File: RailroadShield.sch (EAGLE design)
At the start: 70 parts, among them J1 5520250-3, J2 5520250-3, J3 5520250-3, J4 5520426-4, J5 5520426-4, J6 KK-156-5, J7 KK-156-5, J8 MSTB-02, Q1 PMBT2222, U1 LM393M, U2 MCP2515-ST, U3 MCP2551-SN, U4 MAX3468CSA, U5 MAX3468CSA, U6 MAX3468CSA, U7 LM317LCDR, U8 6N137SD, Y1 16Mhz

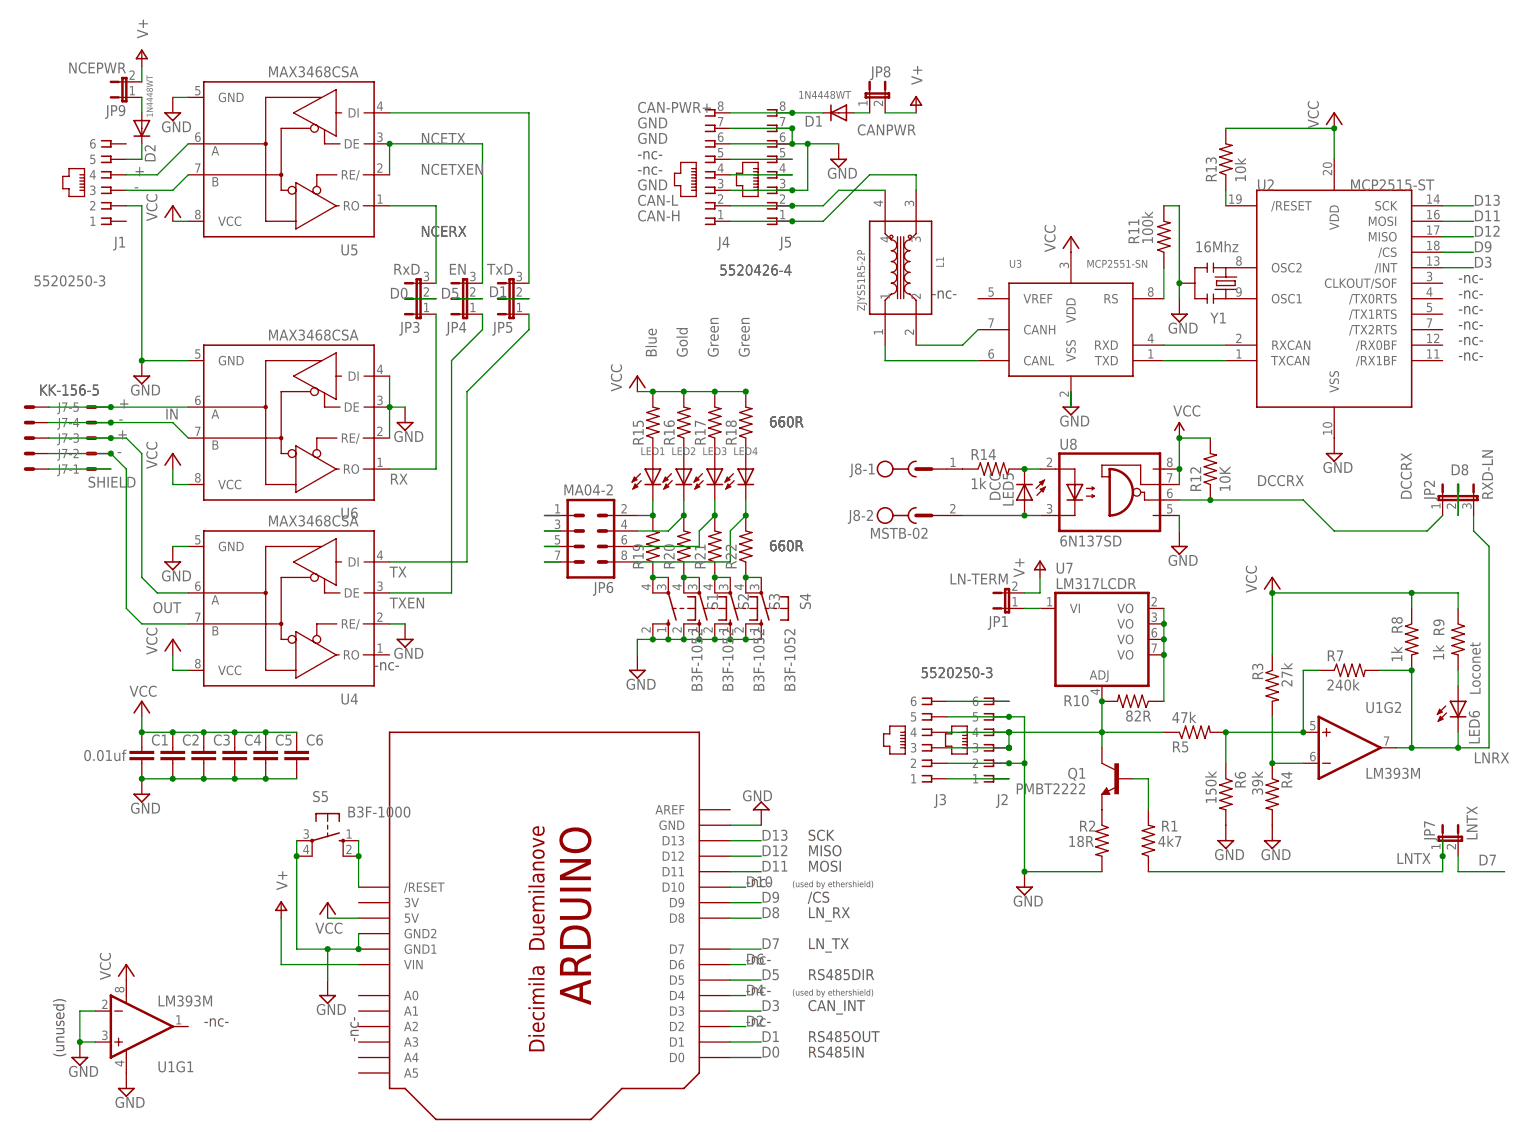
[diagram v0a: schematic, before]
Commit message: 2.3
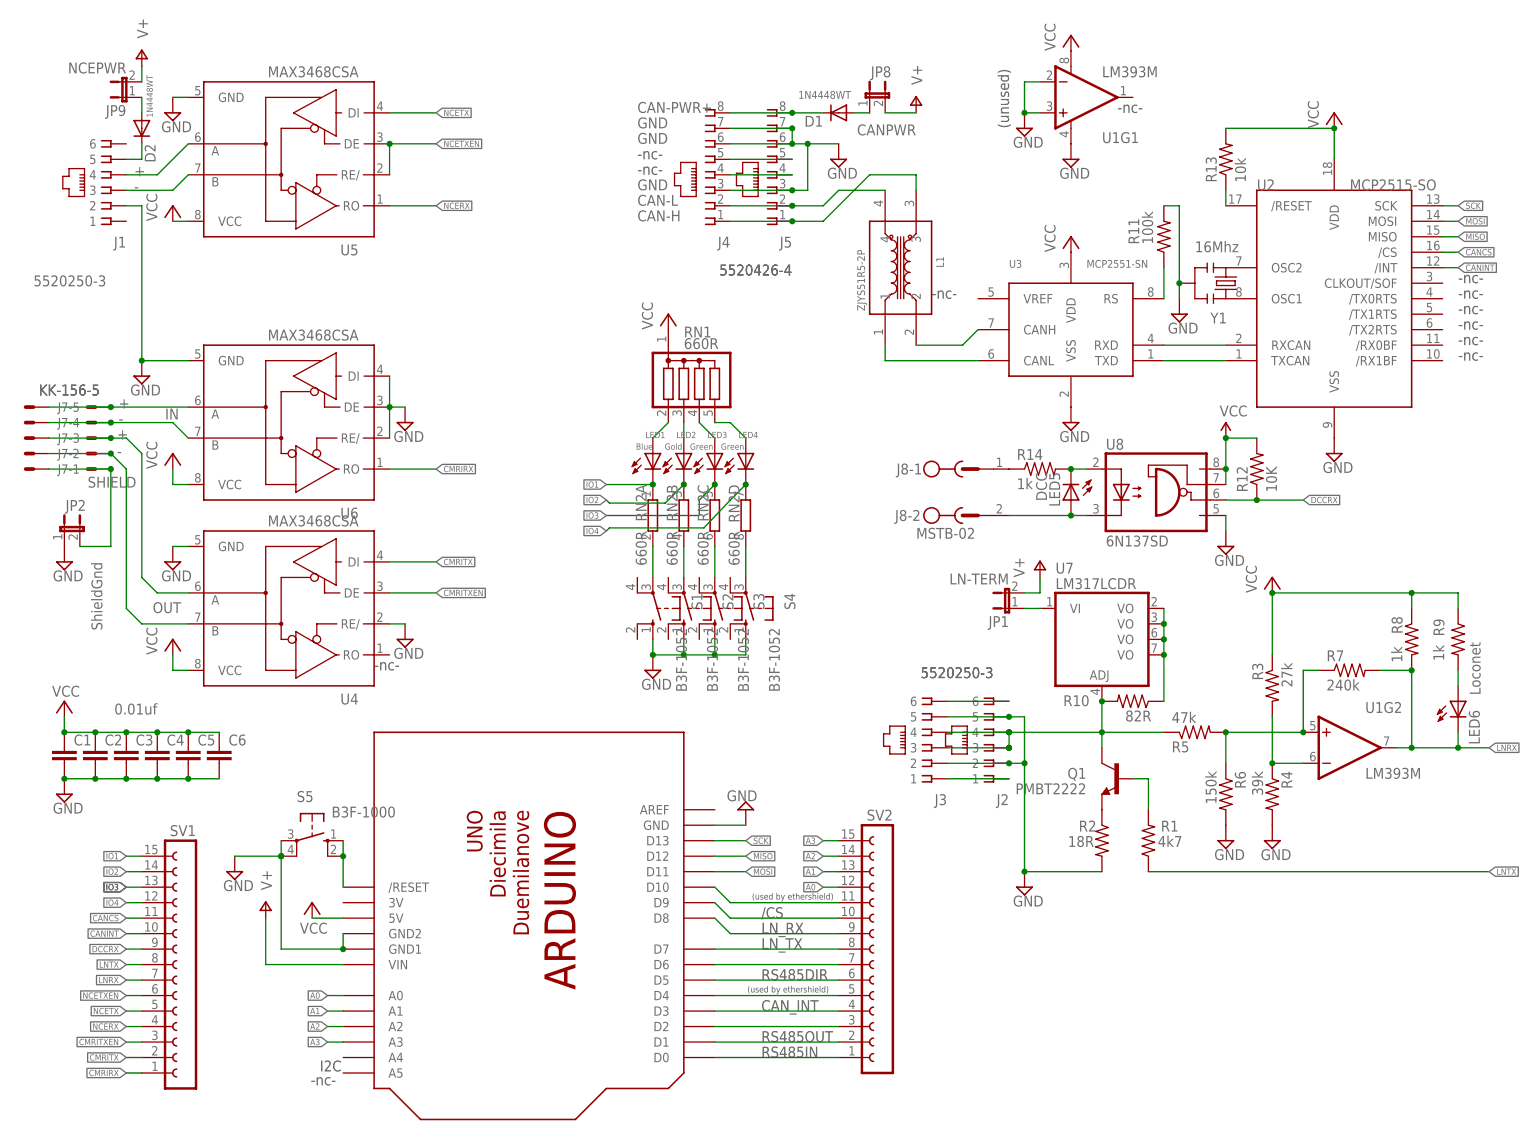
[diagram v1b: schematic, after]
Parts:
- removed JP3: RxD, MCP:JUMPER-3PTH
- removed JP4: EN, MCP:JUMPER-3PTH
- removed JP5: TxD, MCP:JUMPER-3PTH
- removed JP6: MA04-2, MCP:MA04-2
- removed JP7: LNTX, MCP:JUMPER-2PTH_LOCK
- removed R15, R16, R17, R18, R19, R20, R21, R22: 660R, MCP:RESISTOR
- added RN1: 660R, resistor-sil:G04R
- added RN2: 660R, resistor-sil:E4R
- added SV1, SV2: (no value), con-lsta:FE15-1
- D1, D2: device MCP:DIODESOD -> MCP:DIODESOT23
- J1, J2, J3: device MCP:RJ11-6X -> MCP:RJ11-6XRA
- JP2: value RXD-LN -> ShieldGnd; device MCP:JUMPER-3PTH -> MCP:JUMPER-2PTH_LOCK
- U2: value MCP2515-ST -> MCP2515-SO; device MCP:MCP2515-ST -> MCP:MCP2515-SO
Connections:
- net D11 renamed MOSI
- net D12 renamed MISO
- net D13 renamed SCK
- removed net S1+: R19.1, S1.P, S1.P1
- removed net S2+: R20.1, S2.P, S2.P1
- removed net S3+: R21.1, S3.P, S3.P1
- removed net S4+: R22.1, S4.P, S4.P1
- new net A0: SV2.12, U$1.A0
- new net A1: SV2.13, U$1.A1
- new net A2: SV2.14, U$1.A2
- new net A3: SV2.15, U$1.A3
- new net CANCS: SV1.11, U2./CS
- new net CANINT: SV1.10, U2./INT
- new net N$16: RN2A.2, S1.P
- new net N$17: RN2B.2, S2.P
- new net N$18: RN2C.2, S3.P
- new net N$19: RN2D.2, S4.P
- net CMRIRX: now also SV1.1; no longer JP3.1
- net CMRITX: now also SV1.2; no longer JP5.1
- net CMRITXEN: now also SV1.3; no longer JP4.1
- net D0: now also SV2.1; no longer JP3.2
- net D1: now also SV2.2; no longer JP5.2
- net D10: now also SV2.11; no longer JP6.7
- net D2: now also SV2.3; no longer JP6.1
- net D3: now also SV2.4; no longer U2./INT
- net D4: now also SV2.5; no longer JP6.3
- net D5: now also SV2.6; no longer JP4.2
- net D6: now also SV2.7; no longer JP6.5
- net D7: now also SV2.8; no longer JP7.2
- net D8: now also SV2.9; no longer JP2.2
- net D9: now also SV2.10; no longer U2./CS
- net DCCRX: now also SV1.9; no longer JP2.1
- net GND: now also JP2.1; no longer S1.S1, S2.S1, S3.S1, S4.S1
- net IO1: now also RN2A.1, SV1.15; no longer JP6.2, R19.2
- net IO2: now also RN2B.1, SV1.14; no longer JP6.4, R20.2
- net IO3: now also RN2C.1, SV1.13; no longer JP6.6, R21.2
- net IO4: now also RN2D.1, SV1.12; no longer JP6.8, R22.2
- net LNRX: now also SV1.7; no longer JP2.3
- net LNTX: now also SV1.8; no longer JP7.1
- net N$2: now also LED1.A, RN1.2; no longer LED2.A, R16.1
- net N$3: now also LED2.A, RN1.3; no longer LED3.A, R17.1
- net N$4: now also LED3.A, RN1.4; no longer LED4.A, R18.1
- net N$5: now also LED4.A, RN1.5; no longer LED1.A, R15.1
- net N$6: now also JP2.2
- net NCERX: now also SV1.4; no longer JP3.3
- net NCETX: now also SV1.5; no longer JP5.3
- net NCETXEN: now also SV1.6; no longer JP4.3
- net VCC: now also RN1.1; no longer R15.2, R16.2, R17.2, R18.2
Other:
- note added: "2.3"
- note added: "I2C"
- note removed: "2.2"
- note removed: "I/O Test points"
- note removed: "MISO"
- note removed: "MOSI"
- note removed: "RX"
- note removed: "SCK"
- note removed: "TX"
- note removed: "TXEN"
- moved on the sheet: C1, C2, C3, C4, C5, C6, J8-1, J8-2, LED1, LED2, LED3, LED4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
